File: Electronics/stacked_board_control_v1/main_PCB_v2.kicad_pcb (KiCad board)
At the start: 4 copper layers, 100 x 95.5 mm, 188 parts, among them IC202 TJA1057GT/3, IC203 TJA1057GT/3, J201 MEM2075-00-140-01-A, J203 TYPE-C-31-M-12, J204 Conn_02x04_Odd_Even, J205 Conn_ST_STDC14, J207 Conn_01x04, J208 SM02B-GHS-TB_LF__SN_, J209 SM02B-GHS-TB_LF__SN_, J210 SM02B-GHS-TB_LF__SN_, J211 SM02B-GHS-TB_LF__SN_, J212 SM02B-GHS-TB_LF__SN_, J301 Conn_01x02, J302 Conn_01x02, J305 Conn_01x02, J306 Conn_01x02, J307 Conn_01x02, J308 Conn_01x02, J309 Conn_01x02, J310 Conn_01x02, J401 Conn_Coaxial, Q302 DMP3028LFDE, T301 NVMFS4C05NT1G, T302 NVMFS4C05NT1G, U201 STM32H723ZGT6, U202 USBLC6-4SC6, U203 USBLC6-4SC6, U204 BMI270, U206 LIS3MDL, U211 M24C08-FMH6TG, U301 LMR43620MB5RPER, U302 LMR43620MB5RPER, U303 LMR43620MB5RPER, U304 TVS2700DRV, U305 TPS16416DRCR, U401 NRF24L01, U402 RFX2401C, X201 25MHz_Clock, X202 32.768kHz_Clock, Y402 16M

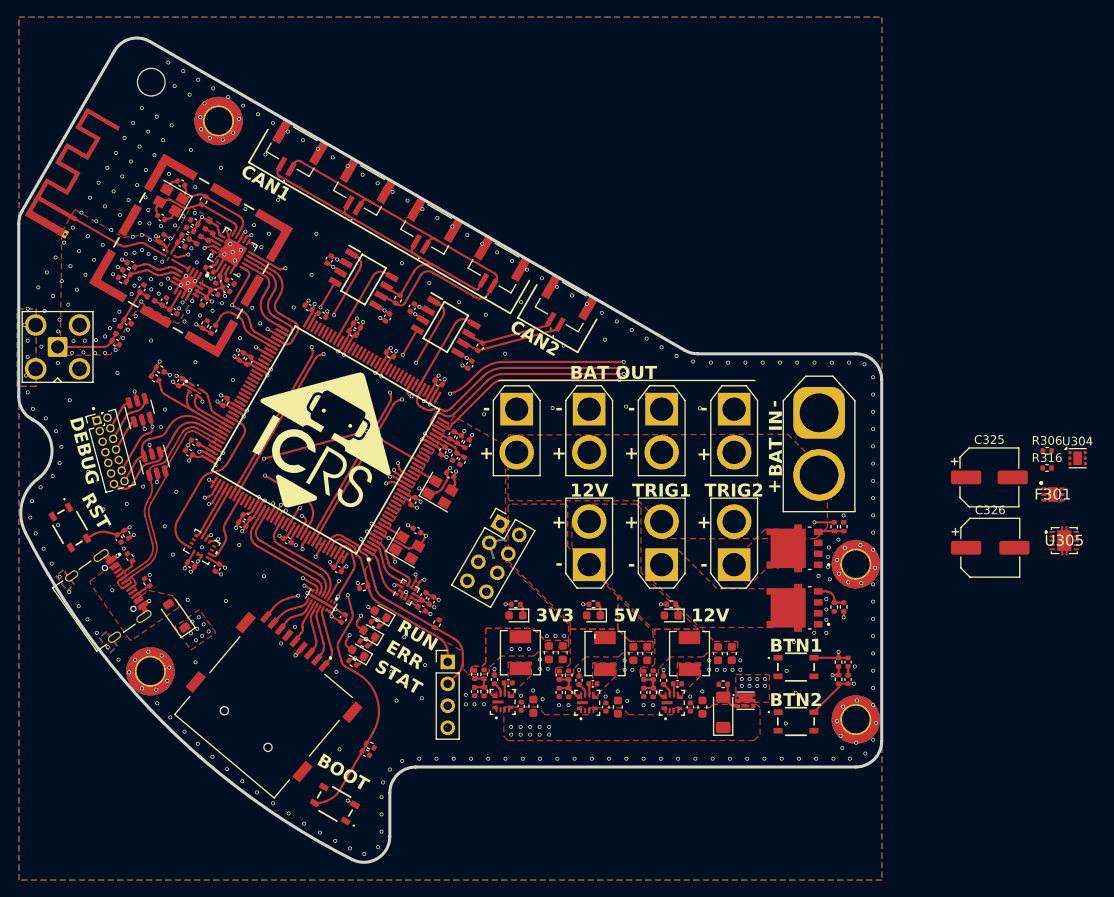
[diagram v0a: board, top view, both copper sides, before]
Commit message: PCBs Done
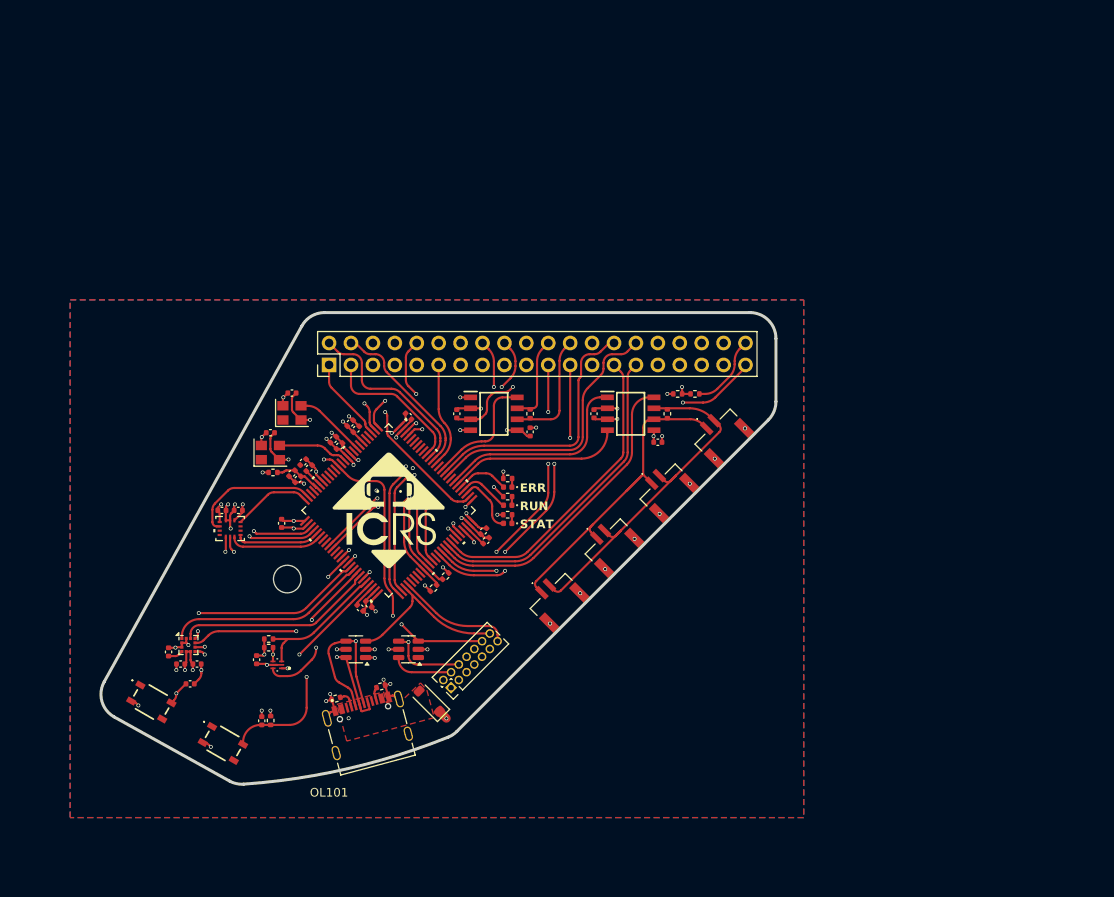
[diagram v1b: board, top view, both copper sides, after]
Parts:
- removed AE401: Antenna, SSL Footprints:Texas_SWRA117D_2.4GHz_Right
- removed C201, C202, C205, C206, C207, C208, C209, C210, C212, C213, C214, C215, C216, C217, C218, C223, C224, C225, C226, C227, C228, C229, C231, C232, C233, C235, C237, C238, C302, C304, C312, C318, C321, C322: 100n, Capacitor_SMD:C_0402_1005Metric
- removed C203, C204, C220, C221, C401, C408: 10n, Capacitor_SMD:C_0402_1005Metric
- removed C211, C219, C222: 10u, Capacitor_SMD:C_0402_1005Metric
- removed C230, C234, C236, C303, C311, C317, C409: 1u, Capacitor_SMD:C_0402_1005Metric
- removed C301, C313, C316: 2u2, Capacitor_SMD:C_0603_1608Metric
- removed C305, C306, C314, C315, C319, C320: 22u, Capacitor_SMD:C_0603_1608Metric
- removed C307, C308, C309: 100p, Capacitor_SMD:C_0402_1005Metric
- removed C310, C323, C324, C406: 1n, Capacitor_SMD:C_0402_1005Metric
- removed C325: 100u, Capacitor_SMD:CP_Elec_6.3x7.7
- removed C326: 100u, Capacitor_SMD:CP_Elec_6.3x5.9
- removed C402, C414, C415, C416, C417: 1p5, Capacitor_SMD:C_0402_1005Metric
- removed C403: 1p, Capacitor_SMD:C_0402_1005Metric
- removed C404: 2n2, Capacitor_SMD:C_0402_1005Metric
- removed C405: 4p7, Capacitor_SMD:C_0402_1005Metric
- removed C407: 33n, Capacitor_SMD:C_0402_1005Metric
- removed C410, C411: 22p, Capacitor_SMD:C_0402_1005Metric
- removed C412: 220p, Capacitor_SMD:C_0402_1005Metric
- removed C413: 0p3, Capacitor_SMD:C_0402_1005Metric
- removed D201: SS0540_R1_00001, Diode_SMD:D_SOD-123
- removed D202: Red, LED_SMD:LED_0603_1608Metric
- removed D203, D301, D302, D304: Green, LED_SMD:LED_0603_1608Metric
- removed D204: Blue, LED_SMD:LED_0603_1608Metric
- removed D303: ZMM10V, Diode_SMD:D_MiniMELF
- removed F301: TPS25961DRVR, SSL Footprints:SON65P200X200X80-7N
- removed FB201: 120R@100MHz, Resistor_SMD:R_0402_1005Metric
- removed FL201: EMIF06-MSD02N16, SSL Footprints:EMIF06MSD02N16
- removed the G*** at (139.6, 91.2)
- removed the G*** at (137.8, 86.6)
- removed IC202, IC203: TJA1057GT/3, SSL Footprints:SOIC127P600X175-8N
- removed J201: MEM2075-00-140-01-A, SSL Footprints:MEM20750014001A
- removed J203: TYPE-C-31-M-12, SSL Footprints:HRO_TYPE-C-31-M-12
- removed J204: Conn_02x04_Odd_Even, Connector_PinHeader_2.54mm:PinHeader_2x04_P2.54mm_Vertical
- removed J205: Conn_ST_STDC14, Connector_PinHeader_1.27mm:PinHeader_2x07_P1.27mm_Vertical
- removed J207: Conn_01x04, Connector_PinHeader_2.54mm:PinHeader_1x04_P2.54mm_Vertical
- removed J208, J209, J210, J211, J212: SM02B-GHS-TB_LF__SN_, SSL Footprints:SM02BGHSTBLFSN
- removed J301: Conn_01x02, Connector_AMASS:AMASS_XT60-M_1x02_P7.20mm_Vertical
- removed J302, J305, J306, J307, J308, J309, J310: Conn_01x02, Connector_AMASS:AMASS_XT30U-F_1x02_P5.0mm_Vertical
- removed J401: Conn_Coaxial, SSL Footprints:SMA_Amphenol_901-143_Horizontal
- removed L301, L303, L305: 4u7, Inductor_SMD:L_Chilisin_BMRA00040420
- removed L401: 3n9, Inductor_SMD:L_0402_1005Metric
- removed L402, L405: 2n4, Inductor_SMD:L_0402_1005Metric
- removed L403: 8n2, Inductor_SMD:L_0402_1005Metric
- removed L404: 2n7, Inductor_SMD:L_0402_1005Metric
- removed Q302: DMP3028LFDE, SSL Footprints:DMP2066UFDE7
- removed R201, R202: 5k1, Resistor_SMD:R_0402_1005Metric
- removed R203, R204, R214, R215, R305: 4k7, Resistor_SMD:R_0402_1005Metric
- removed R205, R206, R207, R210, R304, R314, R315: 10k, Resistor_SMD:R_0402_1005Metric
- removed R208, R209: 120R, Resistor_SMD:R_0402_1005Metric
- removed R211, R212, R213: 2k7, Resistor_SMD:R_0402_1005Metric
- removed R301: 120k, Resistor_SMD:R_0402_1005Metric
- removed R302: 11k, Resistor_SMD:R_0402_1005Metric
- removed R303, R401, R405, R406, R407: 22k, Resistor_SMD:R_0402_1005Metric
- removed R306, R308, R316: 49k9, Resistor_SMD:R_0402_1005Metric
- removed R307: 2k2, Resistor_SMD:R_0402_1005Metric
- removed R309: 12k4, Resistor_SMD:R_0402_1005Metric
- removed R310: 33k, Resistor_SMD:R_0402_1005Metric
- removed R311: 14k3, Resistor_SMD:R_0402_1005Metric
- removed R312, R313: 10R, Resistor_SMD:R_0402_1005Metric
- removed R402: 1M, Resistor_SMD:R_0402_1005Metric
- removed R403, R404: 1k, Resistor_SMD:R_0402_1005Metric
- removed S201, S202, S203, S204: TS20-42-25-WT-160-SMT-TR, SSL Footprints:TS204225WT160SMTTRMSL
- removed S401: SKY13453-385LF, SSL Footprints:SKY13453385LF
- removed SH401: SMS-202F, SSL Footprints:SMS202F
- removed T301, T302: NVMFS4C05NT1G, SSL Footprints:TRANS_NVMFS5834NLWFT1G
- removed U201: STM32H723ZGT6, SSL Footprints:QFP50P2200X2200X160-144N
- removed U202, U203: USBLC6-4SC6, Package_TO_SOT_SMD:SOT-23-6
- removed U204: BMI270, SSL Footprints:BMI270_BOS
- removed U206: LIS3MDL, Package_LGA:LGA-12_2x2mm_P0.5mm
- removed U211: M24C08-FMH6TG, SSL Footprints:M24C08FMH6TG
- removed U301, U302, U303: LMR43620MB5RPER, SSL Footprints:LMR43620MB5RPER_TEX
- removed U304: TVS2700DRV, Package_SON:WSON-6-1EP_2x2mm_P0.65mm_EP1x1.6mm
- removed U305: TPS16416DRCR, SSL Footprints:TPS74901DRCR
- removed U401: NRF24L01, Package_DFN_QFN:QFN-20-1EP_4x4mm_P0.5mm_EP2.5x2.5mm
- removed U402: RFX2401C, SSL Footprints:QFN50P300X300X60-17N-D
- removed X201: 25MHz_Clock, Oscillator:Oscillator_SMD_Abracon_ASE-4Pin_3.2x2.5mm
- removed X202: 32.768kHz_Clock, Oscillator:Oscillator_SMD_Abracon_ASE-4Pin_3.2x2.5mm
- removed Y402: 16M, Oscillator:Oscillator_SMD_Abracon_ASE-4Pin_3.2x2.5mm
- added C101: 100n, Capacitor_SMD:C_0402_1005Metric, F.Cu at (178.1, 91.5)
- added C102: 100n, Capacitor_SMD:C_0402_1005Metric, F.Cu at (154.8, 88.2)
- added C103: 100n, Capacitor_SMD:C_0402_1005Metric, F.Cu at (163.3, 90.3)
- added C104: 100n, Capacitor_SMD:C_0402_1005Metric, F.Cu at (170.7, 88.2)
- added C105: 10n, Capacitor_SMD:C_0402_1005Metric, F.Cu at (123.9, 119.5)
- added C106: 10n, Capacitor_SMD:C_0402_1005Metric, F.Cu at (132.2, 123.8)
- added C109: 100n, Capacitor_SMD:C_0402_1005Metric, F.Cu at (135.7, 85.8)
- added C110: 100n, Capacitor_SMD:C_0402_1005Metric, F.Cu at (133.2, 90.4)
- added C111: 100n, Capacitor_SMD:C_0402_1005Metric, F.Cu at (149.2, 88.5)
- added C112: 100n, Capacitor_SMD:C_0402_1005Metric, F.Cu at (157.9, 101.8)
- added C113: 100n, Capacitor_SMD:C_0402_1005Metric, F.Cu at (141.2, 91.9)
- added C114: 100n, Capacitor_SMD:C_0402_1005Metric, F.Cu at (134.5, 100.9)
- added C115: 100n, Capacitor_SMD:C_0402_1005Metric, F.Cu at (131.6, 116.7)
- added C116: 100n, Capacitor_SMD:C_0402_1005Metric, F.Cu at (143.2, 90.0)
- added C117: 1u, Capacitor_SMD:C_0402_1005Metric, F.Cu at (142.4, 89.3)
- added C118: 100n, Capacitor_SMD:C_0402_1005Metric, F.Cu at (135.7, 95.1)
- added C119: 4u7, Capacitor_SMD:C_0402_1005Metric, F.Cu at (140.5, 91.2)
- added C120: 2u2, Capacitor_SMD:C_0402_1005Metric, F.Cu at (143.6, 110.7)
- added C121: 1u, Capacitor_SMD:C_0402_1005Metric, F.Cu at (136.4, 95.8)
- added C122: 100n, Capacitor_SMD:C_0402_1005Metric, F.Cu at (144.6, 110.3)
- added C123: 2u2, Capacitor_SMD:C_0402_1005Metric, F.Cu at (158.2, 102.9)
- added C124: 1u, Capacitor_SMD:C_0402_1005Metric, F.Cu at (137.7, 94.5)
- added C126: 100n, Capacitor_SMD:C_0402_1005Metric, F.Cu at (137.0, 93.8)
- added C133: 100n, Capacitor_SMD:C_0402_1005Metric, F.Cu at (127.6, 99.4)
- added C134: 100n, Capacitor_SMD:C_0402_1005Metric, F.Cu at (129.5, 99.4)
- added C136: 100n, Capacitor_SMD:C_0402_1005Metric, F.Cu at (121.4, 115.8)
- added C137: 100n, Capacitor_SMD:C_0402_1005Metric, F.Cu at (122.8, 117.2)
- added C138: 1u, Capacitor_SMD:C_0402_1005Metric, F.Cu at (124.7, 117.2)
- added D101: Red, LED_SMD:LED_0402_1005Metric, F.Cu at (160.7, 96.7)
- added D102: Green, LED_SMD:LED_0402_1005Metric, F.Cu at (160.7, 98.8)
- added D103: Blue, LED_SMD:LED_0402_1005Metric, F.Cu at (160.7, 100.9)
- added D104: SS0540_R1_00001, Diode_SMD:D_SOD-123, F.Cu at (151.6, 121.5)
- added FB101: 120R@100MHz, Resistor_SMD:R_0402_1005Metric, F.Cu at (133.5, 95.0)
- added G***: LOGO, SSL Footprints:ICRS_15mm, F.Cu at (147.1, 99.3)
- added G***: LOGO, SSL Footprints:ICRS_30mm, B.Cu at (151.3, 100.6)
- added IC101: TJA1057GT/3, SSL Footprints:SOIC127P600X175-8N, F.Cu at (174.9, 88.2)
- added IC102: TJA1057GT/3, SSL Footprints:SOIC127P600X175-8N, F.Cu at (159.1, 88.2)
- added J101: SM02B-GHS-TB_LF__SN_, SSL Footprints:SM02BGHSTBLFSN, F.Cu at (185.5, 90.8)
- added J102: SM02B-GHS-TB_LF__SN_, SSL Footprints:SM02BGHSTBLFSN, F.Cu at (179.1, 97.1)
- added J103: SM02B-GHS-TB_LF__SN_, SSL Footprints:SM02BGHSTBLFSN, F.Cu at (172.8, 103.5)
- added J104: SM02B-GHS-TB_LF__SN_, SSL Footprints:SM02BGHSTBLFSN, F.Cu at (166.4, 109.8)
- added J108: TYPE-C-31-M-12, SSL Footprints:HRO_TYPE-C-31-M-12, F.Cu at (145.0, 126.4)
- added J110: 20021112-00014T1LF, Connector_PinHeader_1.27mm:PinHeader_2x07_P1.27mm_Vertical, F.Cu at (154.1, 119.9)
- added J112: Conn_02x20_Odd_Even, Connector_PinHeader_2.54mm:PinHeader_2x20_P2.54mm_Vertical, F.Cu at (140.0, 82.5)
- added R101: 120R, Resistor_SMD:R_0402_1005Metric, F.Cu at (179.2, 88.2)
- added R102: 120R, Resistor_SMD:R_0402_1005Metric, F.Cu at (163.3, 88.2)
- added R103: 4k7, Resistor_SMD:R_0402_1005Metric, F.Cu at (133.0, 114.3)
- added R104: 4k7, Resistor_SMD:R_0402_1005Metric, F.Cu at (152.1, 108.4)
- added R105: 10k, Resistor_SMD:R_0402_1005Metric, F.Cu at (133.2, 123.8)
- added R106: 4k7, Resistor_SMD:R_0402_1005Metric, F.Cu at (133.0, 115.3)
- added R107: 100k, Resistor_SMD:R_0402_1005Metric, F.Cu at (182.4, 85.9)
- added R108: 10k, Resistor_SMD:R_0402_1005Metric, F.Cu at (180.4, 85.9)
- added R109: 4k7, Resistor_SMD:R_0402_1005Metric, F.Cu at (153.5, 107.0)
- added R111: 2k7, Resistor_SMD:R_0402_1005Metric, F.Cu at (160.7, 95.7)
- added R112: 2k7, Resistor_SMD:R_0402_1005Metric, F.Cu at (160.7, 97.8)
- added R113: 2k7, Resistor_SMD:R_0402_1005Metric, F.Cu at (160.7, 99.9)
- added R114: 5k1, Resistor_SMD:R_0402_1005Metric, F.Cu at (140.8, 121.2)
- added R115: 5k1, Resistor_SMD:R_0402_1005Metric, F.Cu at (146.0, 119.8)
- added S101: TS20-42-25-WT-160-SMT-TR, SSL Footprints:TS204225WT160SMTTRMSL, F.Cu at (119.4, 121.6)
- added S102: TS20-42-25-WT-160-SMT-TR, SSL Footprints:TS204225WT160SMTTRMSL, F.Cu at (127.7, 126.4)
- added U101: STM32H723VGT6, SSL Footprints:STM32H723VGT6, F.Cu at (146.9, 99.4)
- added U102: M24C08-FMH6TG, SSL Footprints:M24C08FMH6TG, F.Cu at (134.0, 117.3)
- added U103: USBLC6-4SC6, Package_TO_SOT_SMD:SOT-23-6, F.Cu at (143.1, 115.5)
- added U105: USBLC6-4SC6, Package_TO_SOT_SMD:SOT-23-6, F.Cu at (149.2, 115.5)
- added U106: BMI270, SSL Footprints:BMI270_BOS, F.Cu at (128.5, 101.5)
- added U107: LIS3MDL, Package_LGA:LGA-12_2x2mm_P0.5mm, F.Cu at (123.7, 115.0)
- added X101: 25MHz_Clock, Oscillator:Oscillator_SMD_Abracon_ASE-4Pin_3.2x2.5mm, F.Cu at (133.2, 92.7)
- added X102: 32.768kHz_Clock, Oscillator:Oscillator_SMD_Abracon_ASE-4Pin_3.2x2.5mm, F.Cu at (135.7, 88.1)
- OL101: value Main_board_outline_v2 -> ~; footprint SSL Footprints:main_board_outline_v2 -> SSL Footprints:daughter_board_outline_v1
- moved OL101 15.8 mm to (140.0, 80.0)
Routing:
- net /Microcontroller/BTN2: track 92.2 -> 0.00 mm, vias 4 -> 0
- net /Microcontroller/BTN1: track 82.3 -> 0.00 mm, vias 2 -> 0
- net /Microcontroller/TRIG1: track 77.3 -> 0.00 mm, vias 2 -> 0
- net /NRST: track 0.00 -> 74.5 mm, vias 0 -> 4
- net VSYS: track 0.00 -> 69.3 mm, vias 18 -> 1
- net /Microcontroller/TRIG2: track 60.8 -> 0.00 mm, vias 2 -> 0
- net /ISYS_ADC: track 0.00 -> 58.2 mm, vias 0 -> 2
- net /Microcontroller/NRST: track 56.3 -> 0.00 mm, vias 5 -> 0
- net /VSYS_ADC: track 0.00 -> 52.0 mm, vias 0 -> 2
- net GND: track 124.0 -> 73.2 mm, vias 449 -> 47
- net /Microcontroller/CAN1_L: track 49.8 -> 0.00 mm
- net +3.3V: track 92.1 -> 44.9 mm, vias 43 -> 22
- net /USB_DN: track 0.00 -> 42.7 mm, vias 0 -> 2
- net /CAN1_H: track 0.00 -> 41.5 mm
- net /Microcontroller/CAN1_H: track 40.6 -> 0.00 mm
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- removed copper zone on F.Cu, net +12V
- removed copper zone on F.Cu, net +5V
- removed copper zone on F.Cu, net /Power/SW_12V
- removed copper zone on F.Cu, net /Power/SW_3V3
- removed copper zone on F.Cu, net /Power/SW_5V
- removed copper zone on F.Cu, net /Power/TRIG1_D
- removed copper zone on F.Cu, net /Power/TRIG2_D
- removed copper zone on F.Cu, net GND
- removed copper zone on F.Cu, net VBAT
- removed copper zone on In1.Cu, net VBAT
- removed copper zone on In2.Cu, net VBAT
- removed copper zone on F.Cu, net VSYS
- removed copper zone on In2.Cu, net VSYS
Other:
- board size 100 x 95.5 mm -> 78.2 x 54.7 mm
- board text added: "_{IMPERIAL SSL} Control Board v1.0"
- board text removed: "+"
- board text removed: "-"
- board text removed: "12V"
- board text removed: "3V3"
- board text removed: "5V"
- board text removed: "Antenna switch 0: SMA 1: PCB"
- board text removed: "BAT IN"
- board text removed: "BAT OUT"
- board text removed: "BOOT"
- board text removed: "BTN1"
- board text removed: "BTN2"
- board text removed: "Battery voltage: 12-30V"
- board text removed: "CAN1"
- board text removed: "CAN2"
- board text removed: "DEBUG"
- board text removed: "Max current on 3V3, 5V & 12V rails: 2A"
- board text removed: "RST"
- board text removed: "TRIG1"
- board text removed: "TRIG2"
- board text removed: "_{IMPERIAL SSL} Main Board v1.0"
